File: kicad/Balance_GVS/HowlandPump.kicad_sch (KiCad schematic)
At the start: 0 parts

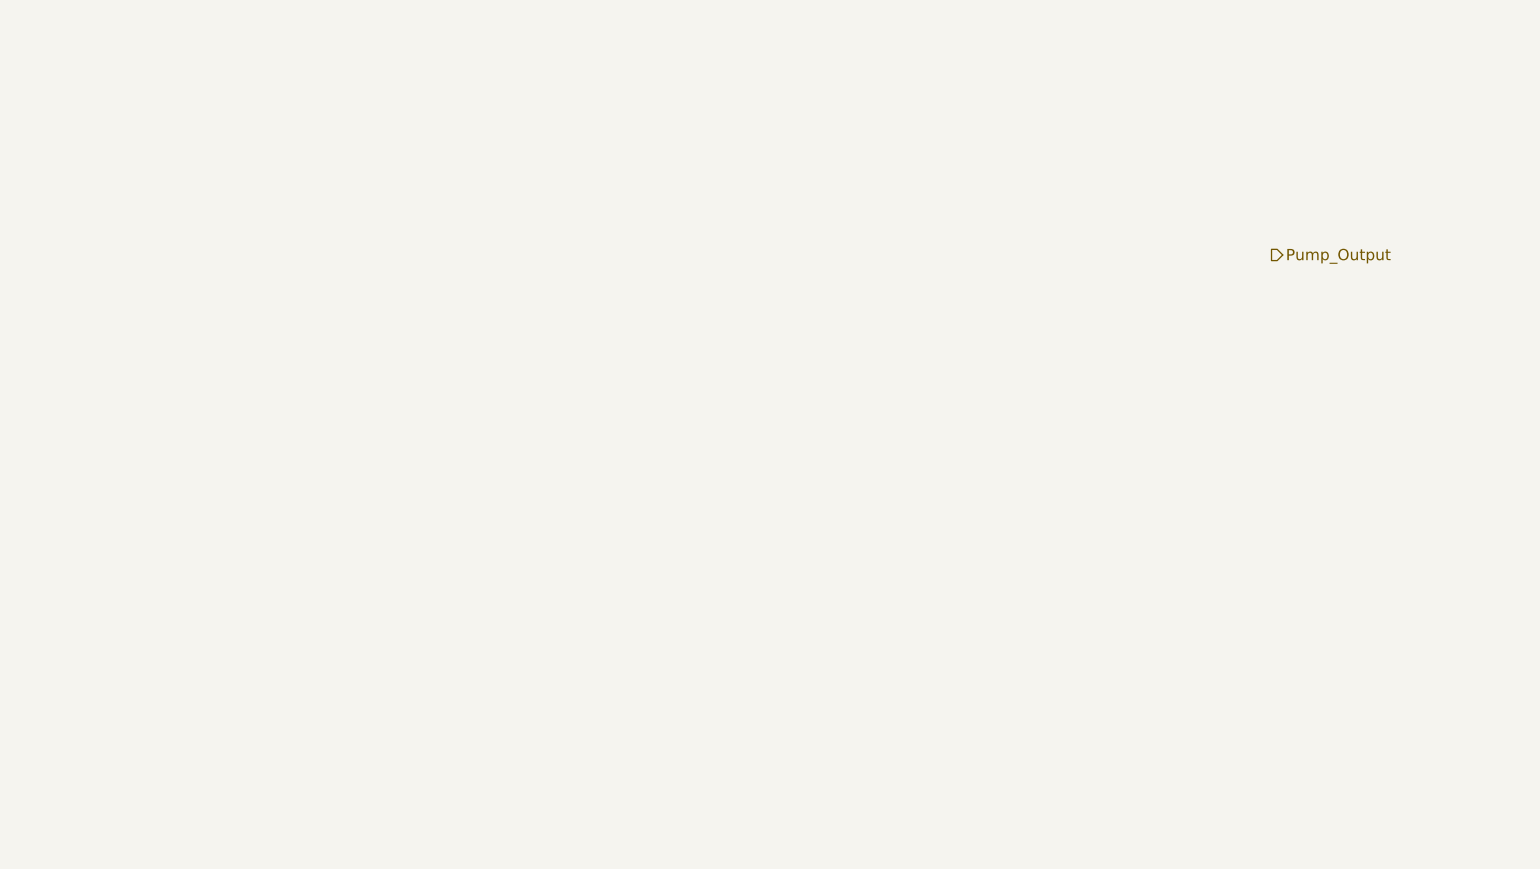
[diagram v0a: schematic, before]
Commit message: Started adding howland connections
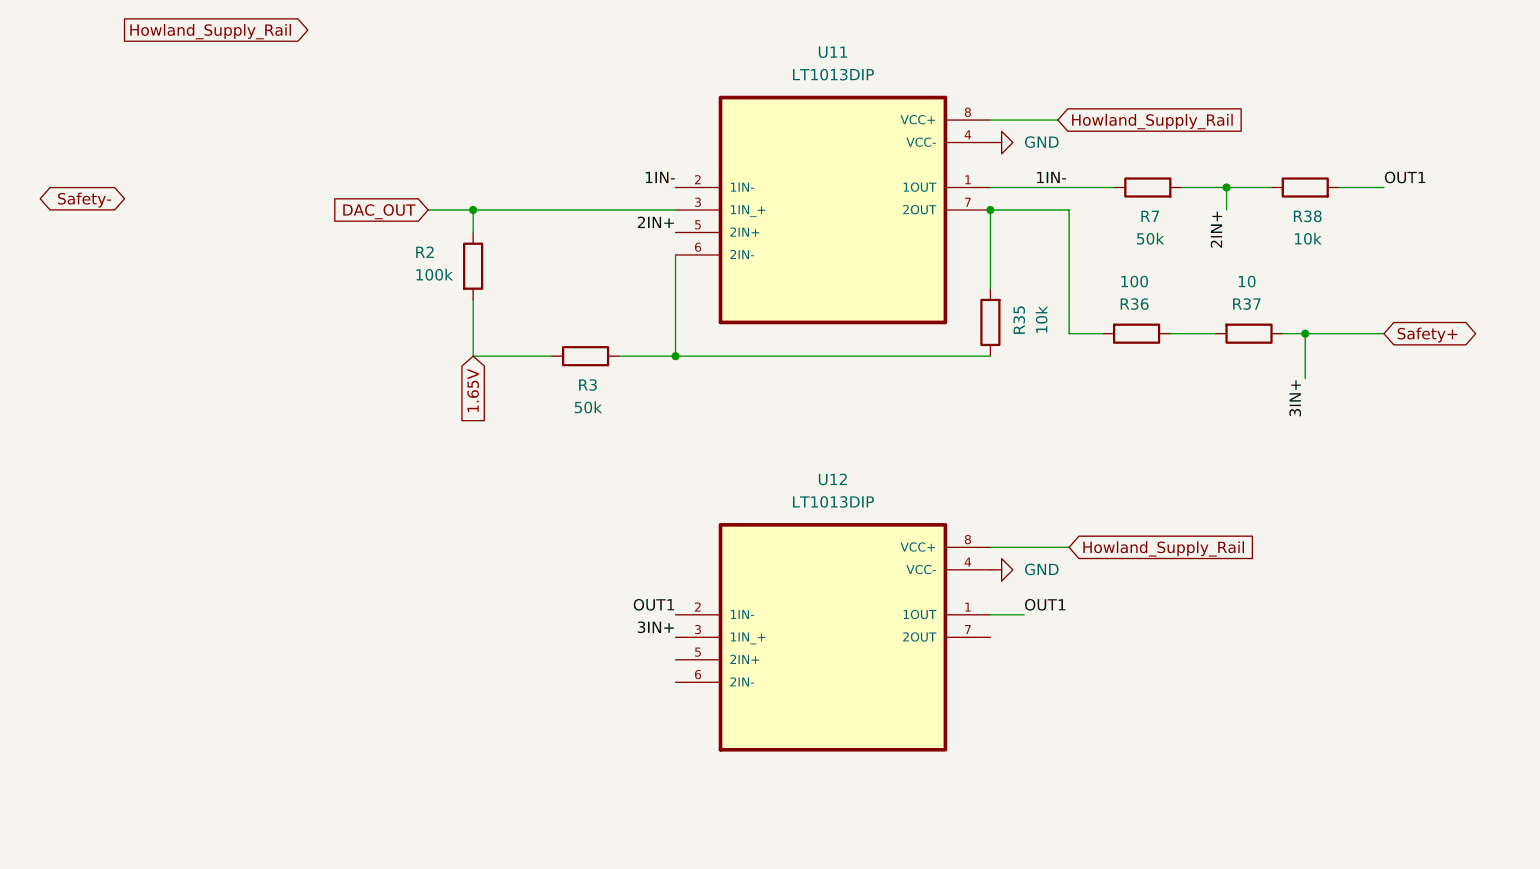
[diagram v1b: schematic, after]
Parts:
- added R2: 100k, symbol Device:R
- added R3, R7: 50k, symbol Device:R
- added R35, R38: 10k, symbol Device:R
- added R36: 100, symbol Device:R
- added R37: 10, symbol Device:R
- added U11, U12: LT1013DIP, LT1013DIP:DIP794W45P254L959H508Q8, symbol LT1013DIP:LT1013DIP
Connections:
- new net: R36.1, R37.2
- new net: R3.2, R35.1, U11.6 (2IN-)
- new net: R35.2, R36.2, U11.7 (2OUT)
- new net 1.65V: R2.2, R3.1
- new net 1IN-: R7.1, U11.1 (1OUT), U11.2 (1IN-)
- new net 2IN+: R38.1, R7.2, U11.5 (2IN+)
- new net DAC_OUT: R2.1, U11.3 (1IN_+)
- new net GND: U11.4 (VCC-), U12.4 (VCC-)
- new net Howland_Supply_Rail: U11.8 (VCC+), U12.8 (VCC+)
- new net OUT1: R38.2, U12.1 (1OUT), U12.2 (1IN-)
- new net Safety+: R37.1, U12.3 (1IN_+)

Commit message: Finish Howland
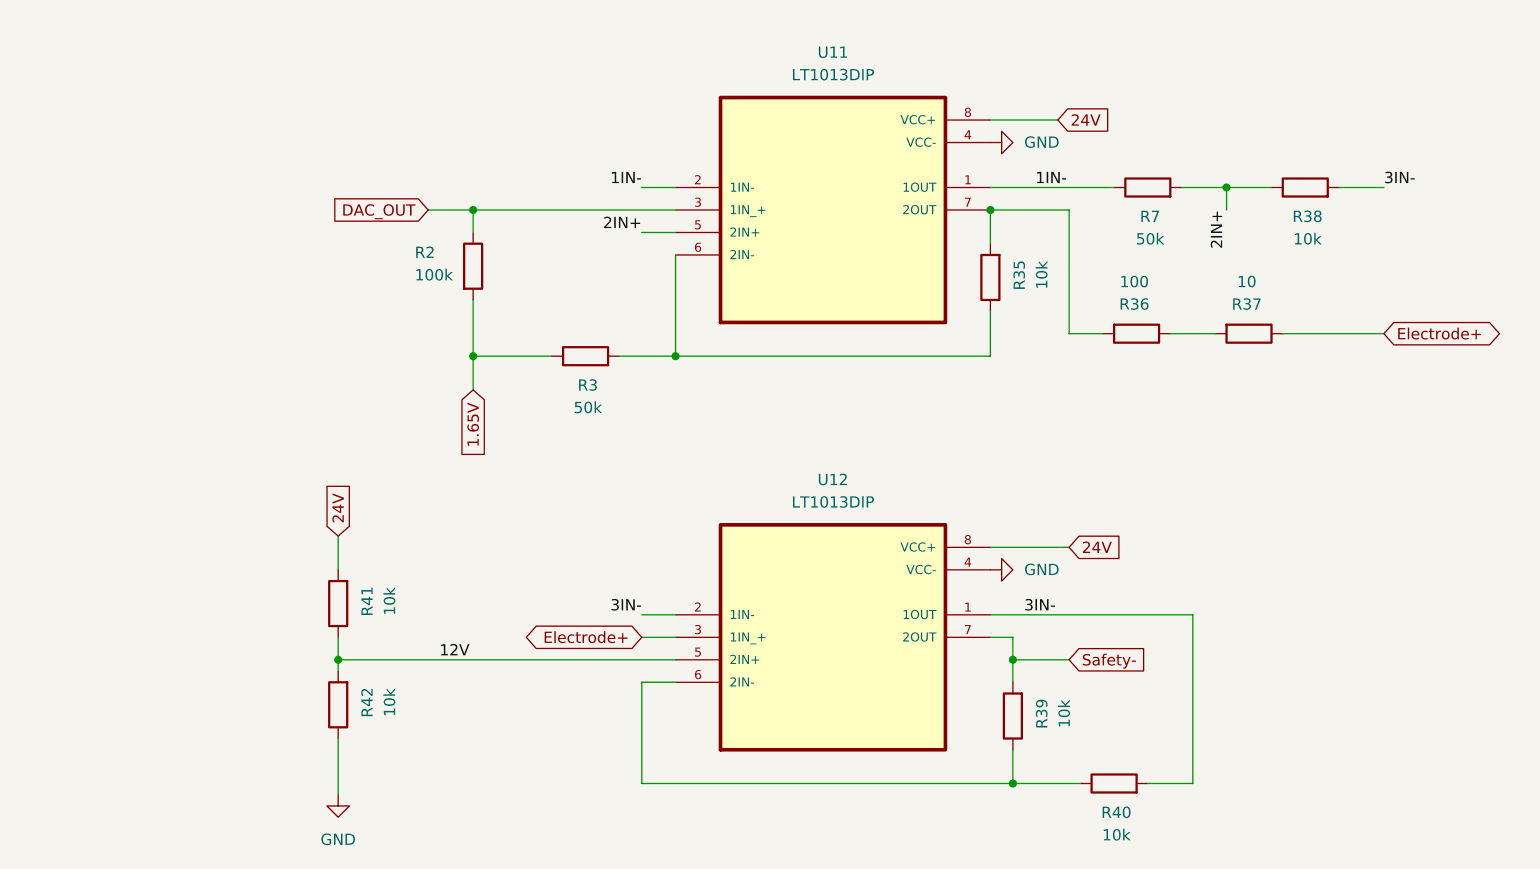
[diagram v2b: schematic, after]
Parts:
- added R39, R40, R41, R42: 10k, symbol Device:R
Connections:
- net GND: now also R42.1
- net Safety-: now also U12.7 (2OUT), R39.2
- net 12V: now reaches U12.5 (2IN+)
- net 12V: now also R41.1, R42.2
- net at U12.6 (2IN-): now also R39.1, R40.1
- net Howland_Supply_Rail renamed 24V
- net 24V: now also R41.2
- net OUT1 renamed 3IN-
- net 3IN-: now also R40.2
- net Safety+ renamed Electrode+
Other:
- moved on the sheet: R35
